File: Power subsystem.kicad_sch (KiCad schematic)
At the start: 17 parts, among them J1 Conn_01x02_Pin, J2 Conn_01x04_Pin, P1 USB_C_Plug, U1 INA219AxD, U3 TP4056-42-ESOP8

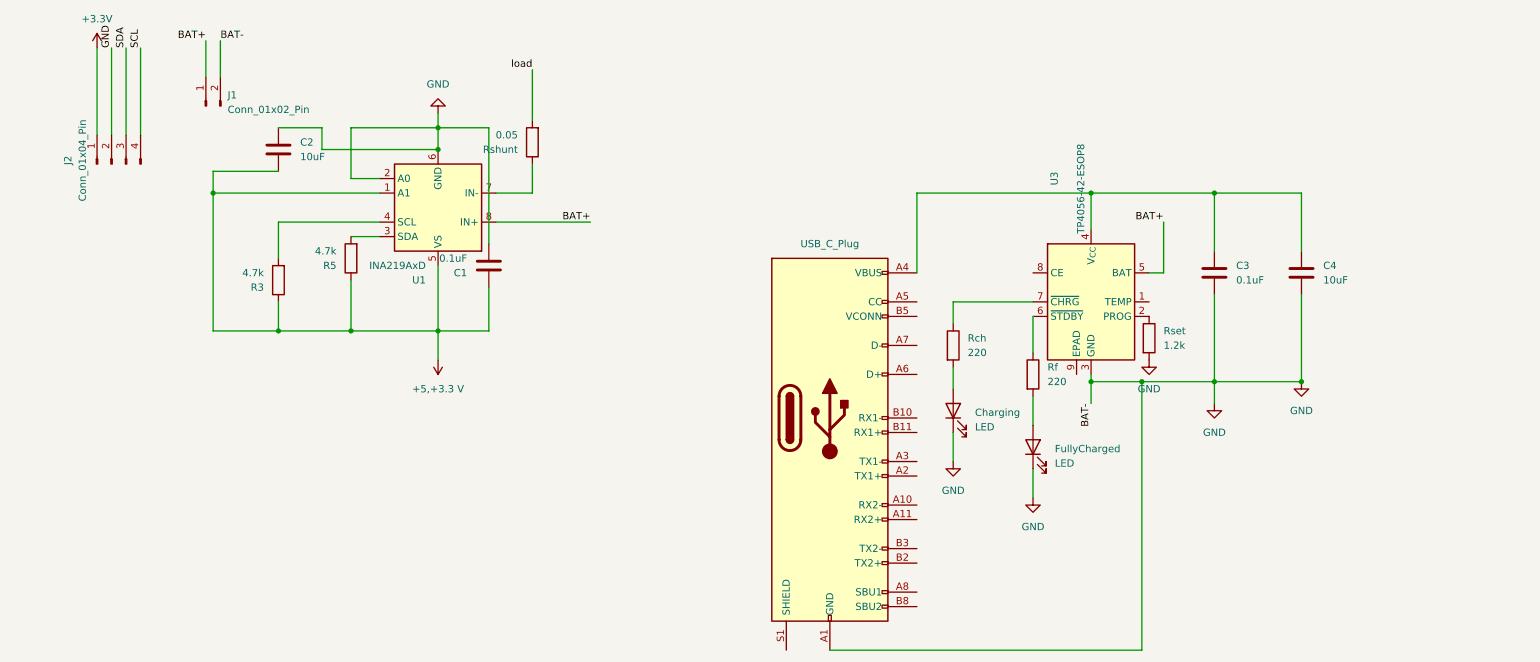
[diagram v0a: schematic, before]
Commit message: Add files via upload
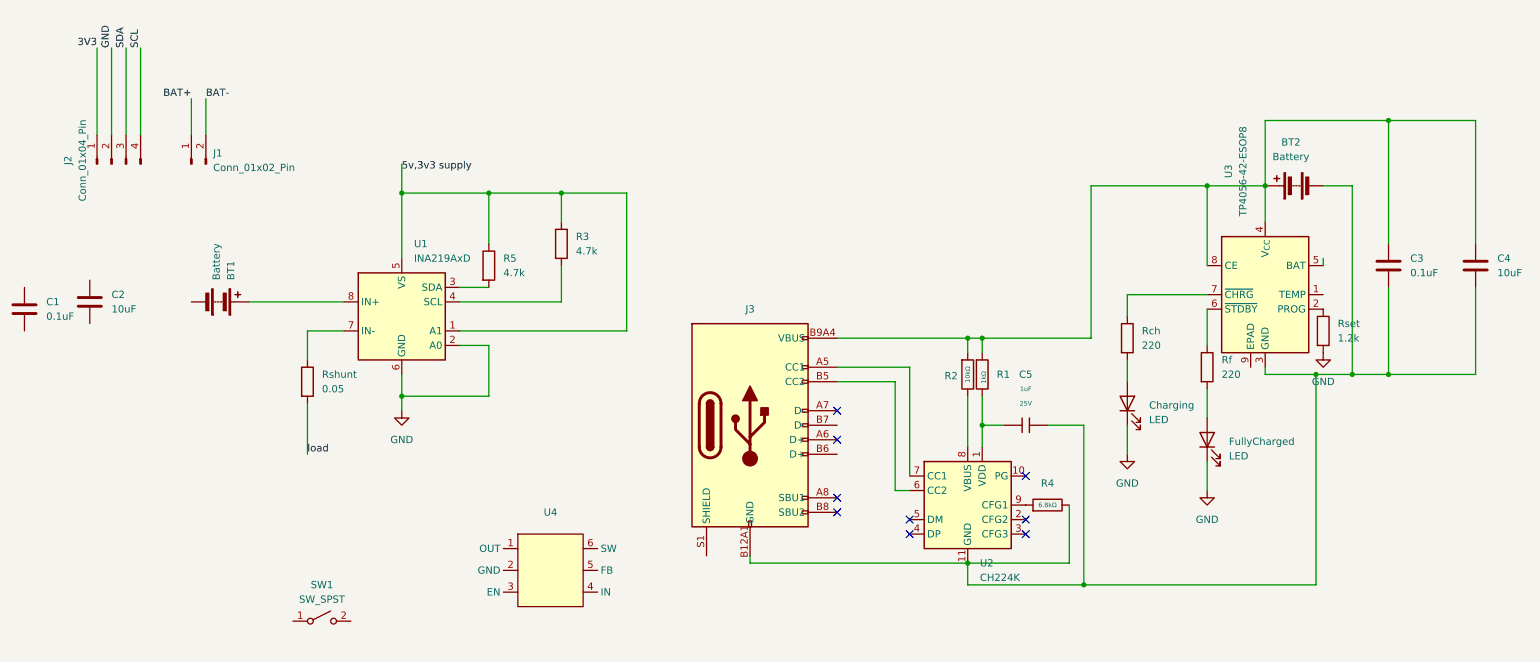
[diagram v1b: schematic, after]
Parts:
- removed P1: USB_C_Plug, symbol Connector:USB_C_Plug
- added BT1, BT2: Battery, symbol Device:Battery
- added C5: 1uF, PCM_JLCPCB:C_0402, symbol JLCPCB-Capacitors:0402,1uF
- added J3: Connector, USB-TYPE-C-16P, PCM_JLCPCB:TYPE-C-SMD_HX-TYPE-C-16PIN, symbol JLCPCB-Extended:Connector, USB-TYPE-C-16P
- added R1: 1kΩ, PCM_JLCPCB:R_0603, symbol JLCPCB-Resistors:0603,1kΩ
- added R2: 10kΩ, PCM_JLCPCB:R_0603, symbol JLCPCB-Resistors:0603,10kΩ
- added R4: 6.8kΩ, PCM_JLCPCB:R_0603, symbol JLCPCB-Resistors:0603,6.8kΩ
- added SW1: SW_SPST, symbol Switch:SW_SPST
- added U2: CH224K, Package_SO:SSOP-10-1EP_3.9x4.9mm_P1mm_EP2.1x3.3mm, symbol Interface_USB:CH224K
- added U4: ~, ETA1038:Untitled, symbol ETA1038:ETA1038
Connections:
- net BAT+: no longer U1.8 (IN+), U3.5 (BAT)
- net GND: no longer C1.2, C2.1, C3.2, C4.2, J1.2 (Pin_2), U3.3 (GND)
- net at C3.1, C4.1, U3.4 (V_{CC}): now also U3.8 (CE), BT2.1 (+), J3.A9B4 (VBUS), J3.B9A4 (VBUS), R1.1, R2.1
- net +3.3V renamed 3V3
- net +5,+3.3 V renamed 5v,3v3 supply
- net 5v,3v3 supply: no longer C1.1, C2.2
- new net: BT2.2 (-), C3.2, C4.2, C5.2, J3.A12B1 (GND), J3.B12A1 (GND), R4.2, U2.11 (GND), U3.3 (GND)
- new net: J3.A5 (CC1), U2.7 (CC1)
- new net: J3.B5 (CC2), U2.6 (CC2)
- new net: BT1.1 (+), U1.8 (IN+)
- new net: R4.1, U2.9 (CFG1)
- new net: C5.1, R1.2, U2.1 (VDD)
- new net: R2.2, U2.8 (VBUS)
- new net BAT-: J1.2 (Pin_2)
- no-connect marks 0 -> 9
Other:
- moved on the sheet: C1, C2, C3, C4, Charging, FullyCharged, J1, R3, R5, Rch, Rf, Rset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

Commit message: Add files via upload
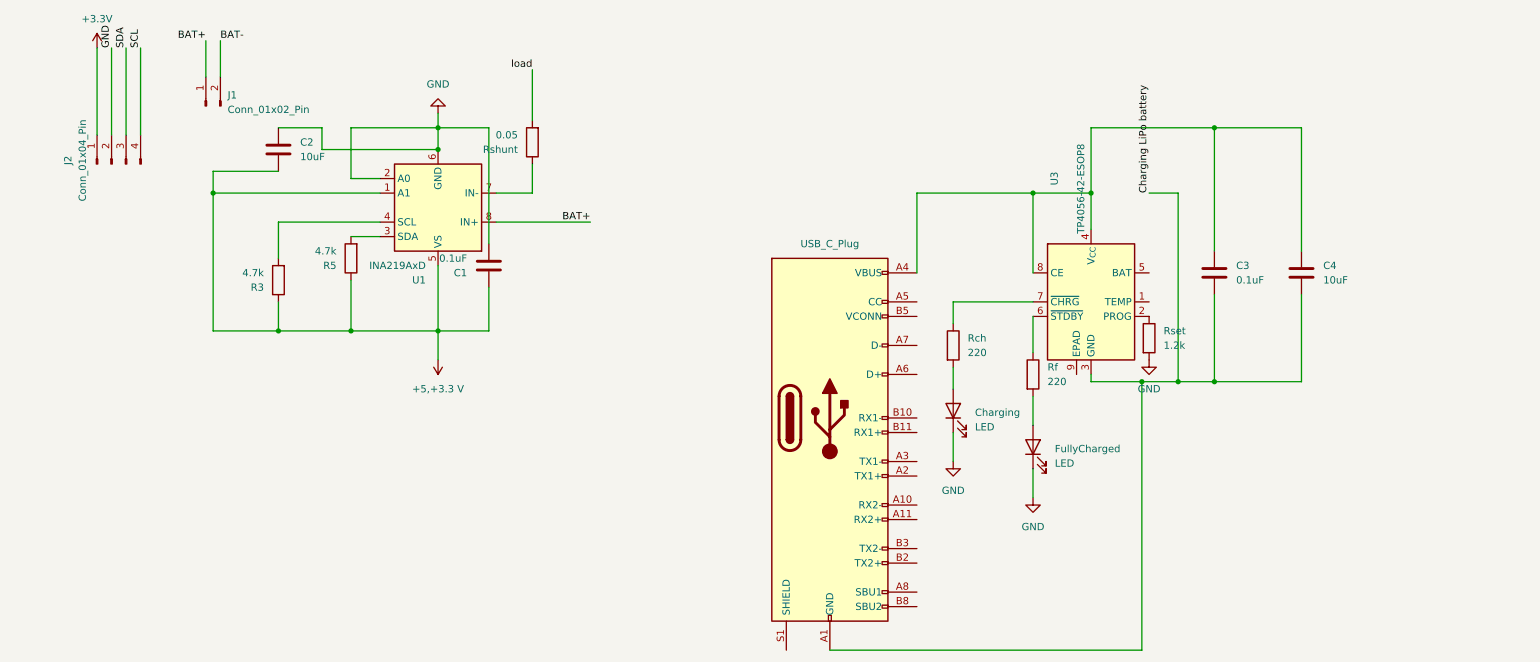
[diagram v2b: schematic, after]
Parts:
- removed BT1, BT2: Battery, symbol Device:Battery
- removed C5: 1uF, PCM_JLCPCB:C_0402, symbol JLCPCB-Capacitors:0402,1uF
- removed J3: Connector, USB-TYPE-C-16P, PCM_JLCPCB:TYPE-C-SMD_HX-TYPE-C-16PIN, symbol JLCPCB-Extended:Connector, USB-TYPE-C-16P
- removed R1: 1kΩ, PCM_JLCPCB:R_0603, symbol JLCPCB-Resistors:0603,1kΩ
- removed R2: 10kΩ, PCM_JLCPCB:R_0603, symbol JLCPCB-Resistors:0603,10kΩ
- removed R4: 6.8kΩ, PCM_JLCPCB:R_0603, symbol JLCPCB-Resistors:0603,6.8kΩ
- removed SW1: SW_SPST, symbol Switch:SW_SPST
- removed U2: CH224K, Package_SO:SSOP-10-1EP_3.9x4.9mm_P1mm_EP2.1x3.3mm, symbol Interface_USB:CH224K
- removed U4: ~, ETA1038:Untitled, symbol ETA1038:ETA1038
- added P1: USB_C_Plug, symbol Connector:USB_C_Plug
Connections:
- net 5v,3v3 supply is gone; now on net +5,+3.3 V: R3.1, R5.1, U1.1 (A1), U1.5 (VS)
- net BAT+: now also U1.8 (IN+)
- net GND: now also C1.2, C2.1
- net Charging LiPo battery: now reaches C3.2, C4.2, U3.3 (GND)
- net Charging LiPo battery: now also P1.A1 (GND), P1.A12 (GND), P1.B1 (GND), P1.B12 (GND)
- net at C3.1, C4.1, U3.4 (V_{CC})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: now also P1.A4 (VBUS), P1.A9 (VBUS), P1.B4 (VBUS), P1.B9 (VBUS)
- net +5,+3.3 V: now reaches C2.2
- net +5,+3.3 V: now also C1.1
- net 3V3 renamed +3.3V
- no-connect marks 9 -> 0
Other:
- moved on the sheet: C1, C2, C3, C4, Charging, FullyCharged, J1, R3, R5, Rch, Rf, Rset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
